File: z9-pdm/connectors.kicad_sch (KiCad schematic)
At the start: 11 parts, among them J10 RedCubeTerminal, J11 RedCubeTerminal, J12 Wago 12 pin 1 level 3.5mm 260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, J13 TE_DT15-12PC-B016 -Conn_01x12, J16 JST GH, J17 Wago 12 pin 1 level 3.5mm 260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, J19 Wago 12 pin 1 level 3.5mm 260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, J2 TE_DT15-12PC-B016 -Conn_01x12, J20 TE_DT15-12PC-B016 -Conn_01x12, J21 Wago 12 pin 1 level 3.5mm 260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, J22 TE_DT15-12PC-B016 -Conn_01x12

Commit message: x
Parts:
- J16: symbol dnt_global:JST_06 -> dnt_global:Conn_JST_06
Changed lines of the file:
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@@
 	)
 	(symbol
-		(lib_id "dnt_global:JST_06")
+		(lib_id "dnt_global:Conn_JST_06")
 		(at 67.31 167.64 0)
 		(mirror x)

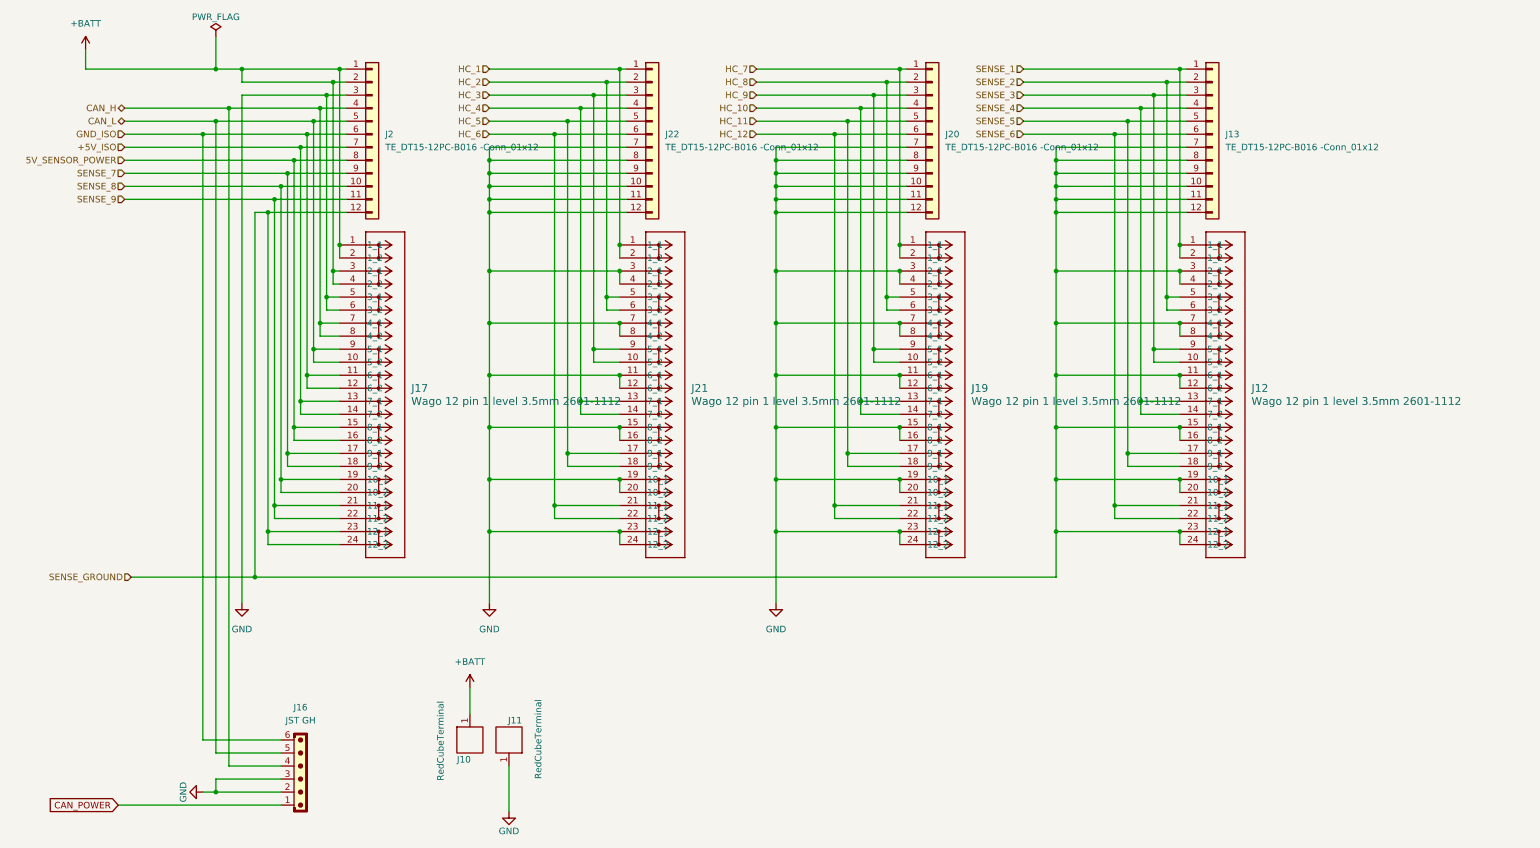
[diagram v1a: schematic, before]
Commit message: x
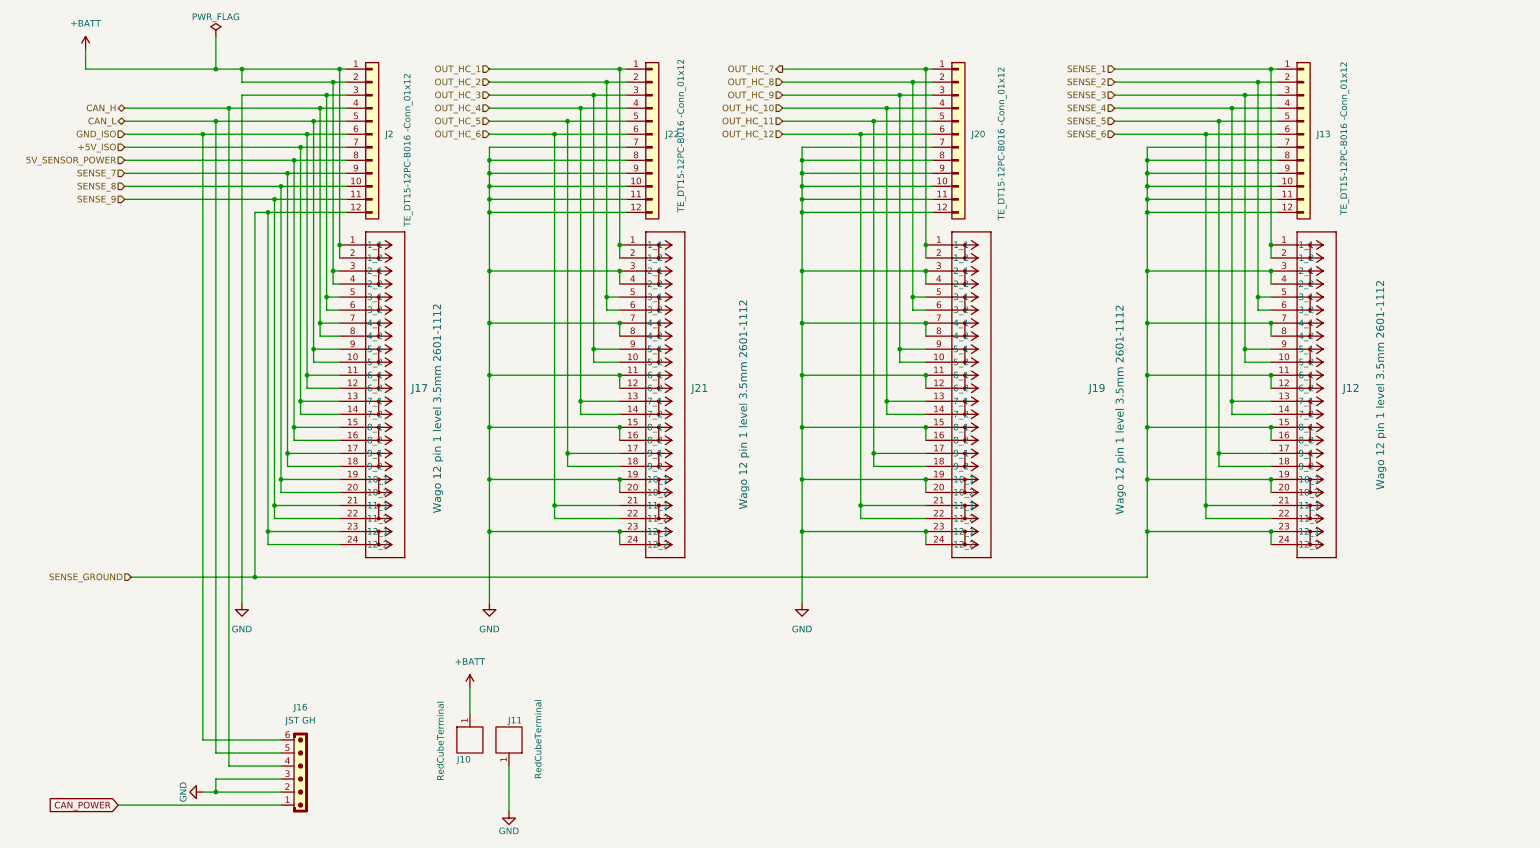
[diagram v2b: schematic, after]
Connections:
- net HC_1 renamed OUT_HC_1
- net HC_10 renamed OUT_HC_10
- net HC_11 renamed OUT_HC_11
- net HC_12 renamed OUT_HC_12
- net HC_2 renamed OUT_HC_2
- net HC_3 renamed OUT_HC_3
- net HC_4 renamed OUT_HC_4
- net HC_5 renamed OUT_HC_5
- net HC_6 renamed OUT_HC_6
- net HC_7 renamed OUT_HC_7
- net HC_8 renamed OUT_HC_8
- net HC_9 renamed OUT_HC_9
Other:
- moved on the sheet: J12, J13, J19, J20
